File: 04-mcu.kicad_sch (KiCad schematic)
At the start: 16 parts, among them J4 USB-C, J5 microSD_PushPush, SW1 RESET, SW2 BOOT, U6 ESP32-S3-WROOM-1-N8R2

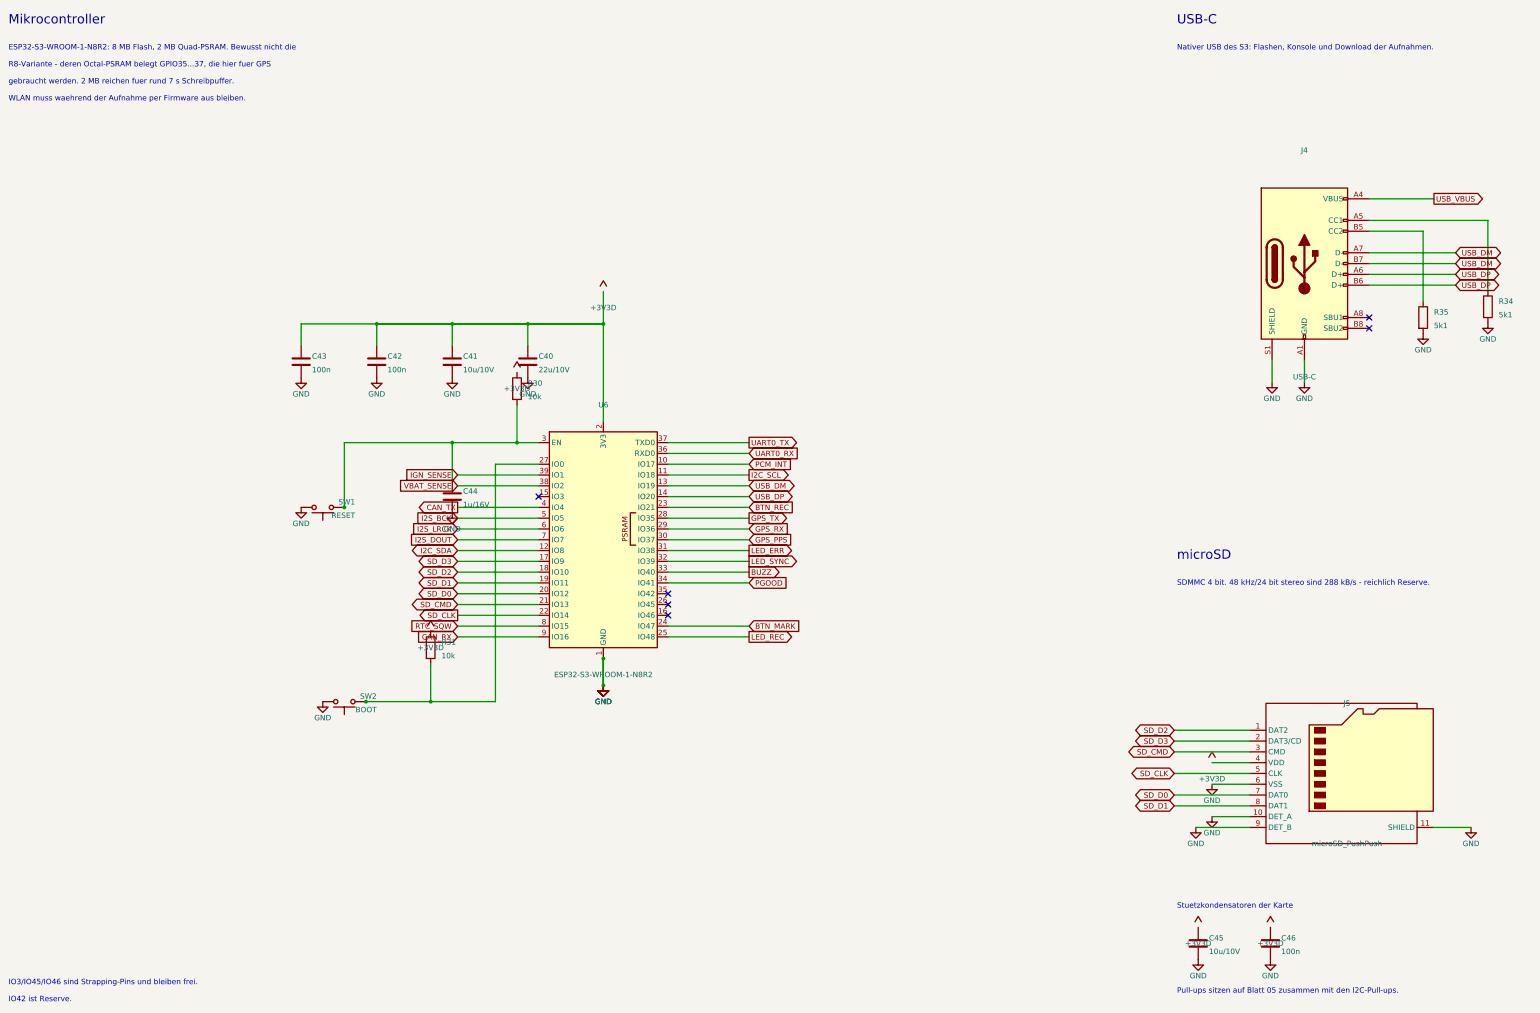
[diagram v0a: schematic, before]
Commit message: modified:   01-power.kicad_sch 	modified:   02-analog.kicad_sch 	modified:   03-adc.kicad_sch 	modified:   04-mcu.kicad_sch 	modified:   05-io.kicad_sch 	modified:   exhaust-mic.kicad_pcb 	modified:   exhaust-mic.kicad_pro 	modified:   exhaust-mic.kicad_sch 	modified:   mic-head/mic-head.kicad_pcb 	modified:   mic-head/mic-head.kicad_pro 	modified:   mic-head/mic-head.kicad_sch 	new file:   ~exhaust-mic.kicad_pro.lck
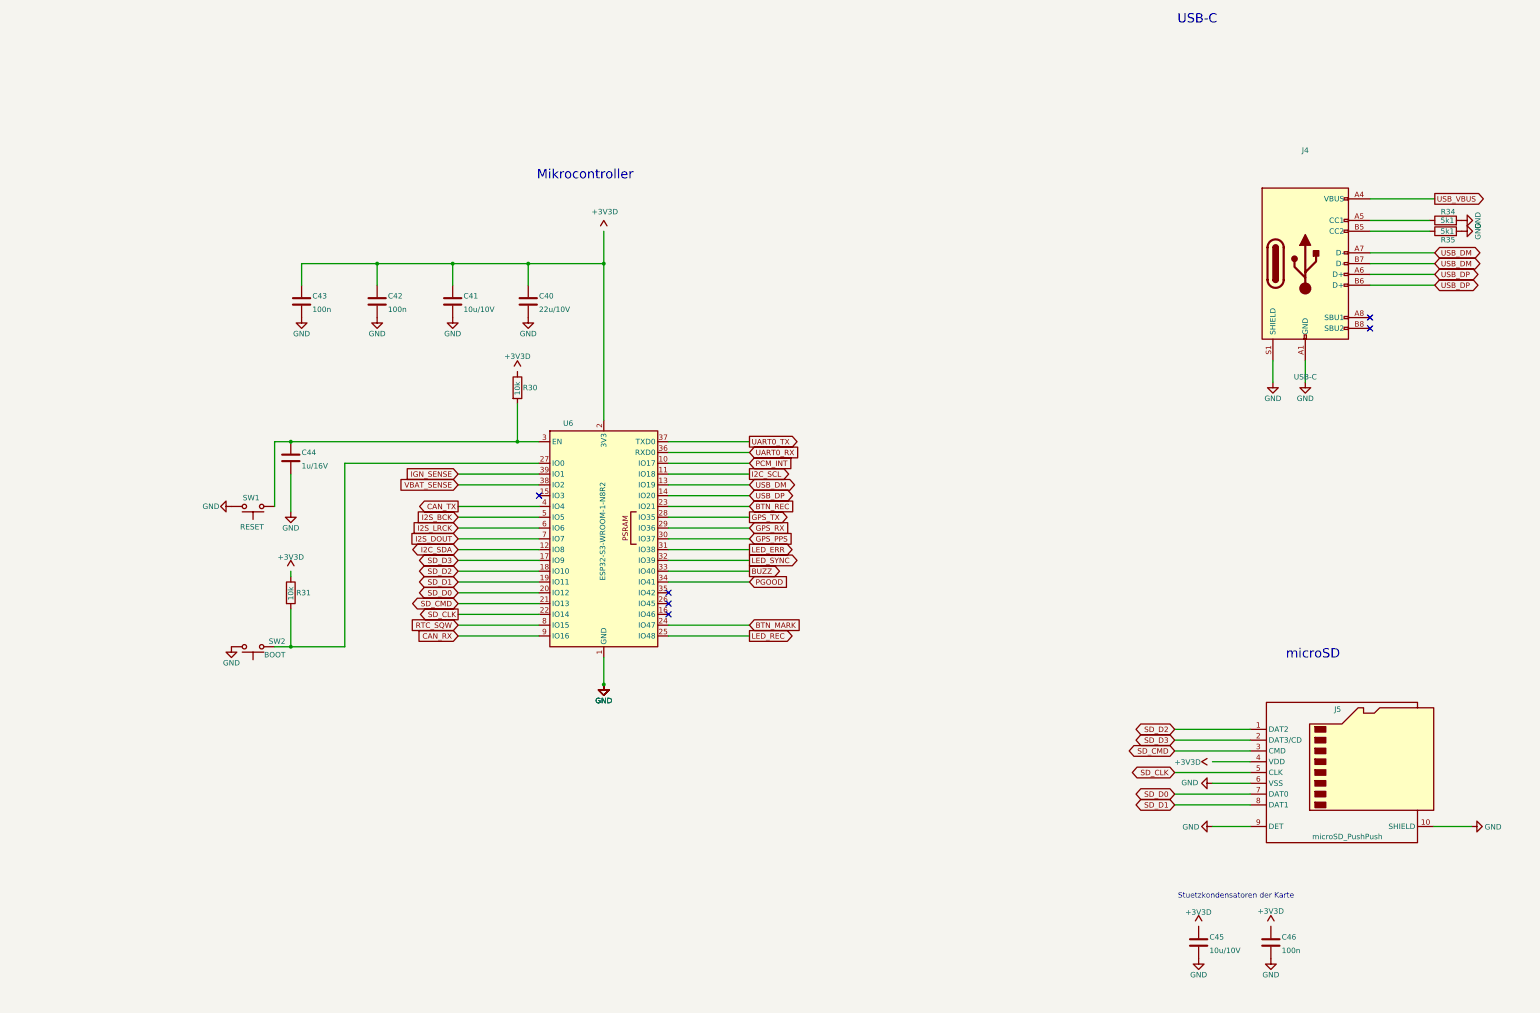
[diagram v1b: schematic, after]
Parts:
- removed J5: microSD_PushPush, Connector_Card:microSD_HC_Hirose_DM3D-SF, symbol Connector:Micro_SD_Card_Det2
- added J5: microSD_PushPush, Connector_Card:microSD_HC_Hirose_DM3D-SF, symbol Connector:Micro_SD_Card_Det1
- U6: footprint RF_Module:ESP32-S3-WROOM-1 -> RF_Module:ESP32-S2-WROOM
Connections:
- net +3V3D: now also J5.4 (VDD)
- net GND: now also J5.10 (SHIELD), J5.6 (VSS), J5.9 (DET)
- net SD_CLK: now also J5.5 (CLK)
- net SD_CMD: now also J5.3 (CMD)
- net SD_D0: now also J5.7 (DAT0)
- net SD_D1: now also J5.8 (DAT1)
- net SD_D2: now also J5.1 (DAT2)
- net SD_D3: now also J5.2 (DAT3/CD)
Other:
- note removed: "ESP32-S3-WROOM-1-N8R2: 8 MB Flash, 2 MB Quad-PSRAM. Bewusst nicht die"
- note removed: "IO3/IO45/IO46 sind Strapping-Pins und bleiben frei."
- note removed: "IO42 ist Reserve."
- note removed: "Nativer USB des S3: Flashen, Konsole und Download der Aufnahmen."
- note removed: "Pull-ups sitzen auf Blatt 05 zusammen mit den I2C-Pull-ups."
- note removed: "R8-Variante - deren Octal-PSRAM belegt GPIO35...37, die hier fuer GPS"
- note removed: "SDMMC 4 bit. 48 kHz/24 bit stereo sind 288 kB/s - reichlich Reserve."
- note removed: "WLAN muss waehrend der Aufnahme per Firmware aus bleiben."
- note removed: "gebraucht werden. 2 MB reichen fuer rund 7 s Schreibpuffer."
- company: Hayabusa / exhaust-mic -> (none)
- title: Exhaust-Mic - ESP32-S3, USB-C und microSD -> ESP32-S3, USB-C und microSD
- moved on the sheet: C40, C41, C42, C43, C44, R31, R34, R35, SW1, SW2
